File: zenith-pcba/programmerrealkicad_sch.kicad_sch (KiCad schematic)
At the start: 19 parts, among them SW1 G4R152312, U1 XC7K70T-FBG676, U3 CH347T, U4 AP63203WU, X1 SX5B8.000F1520F30

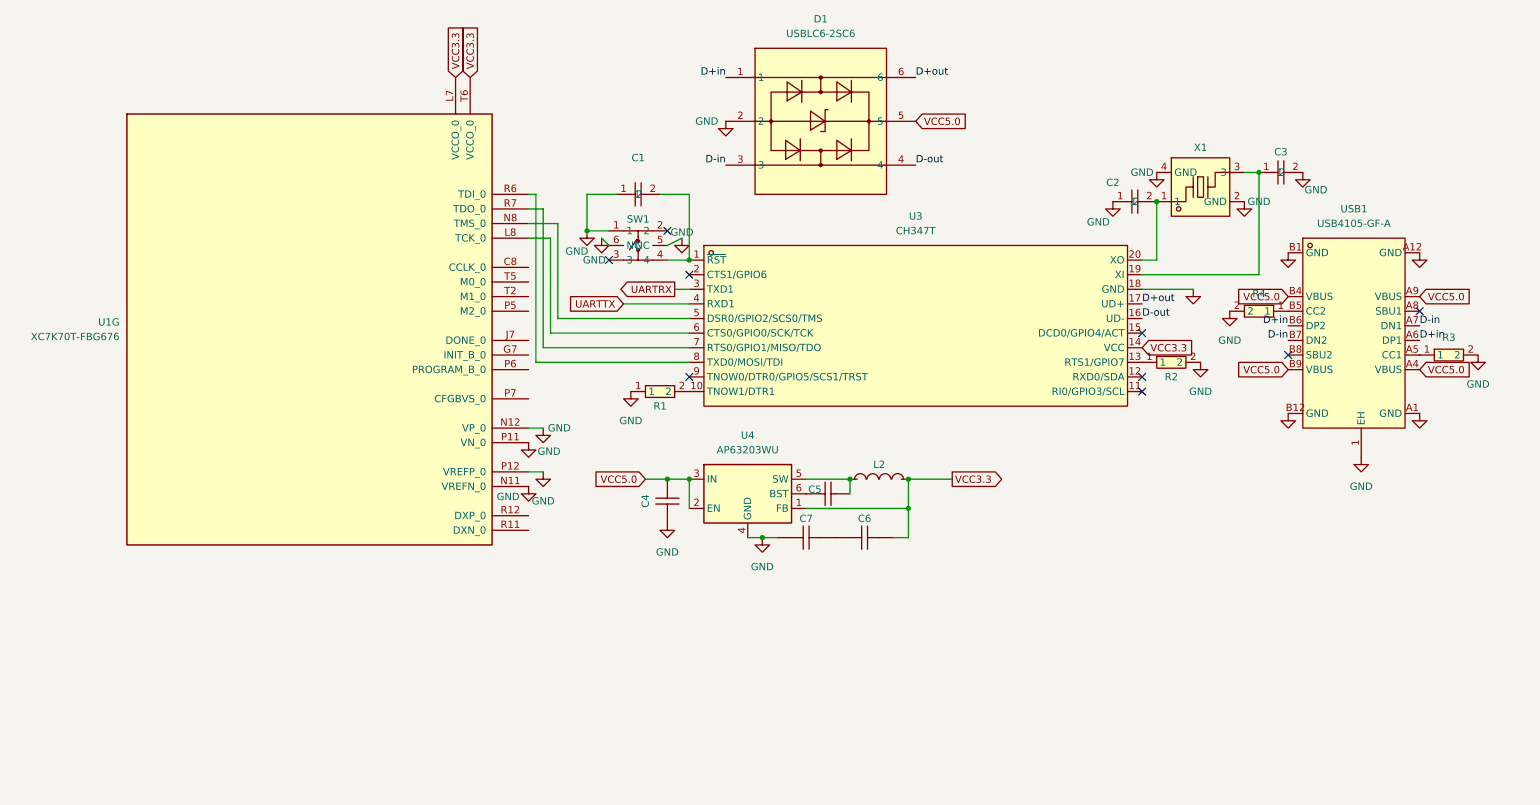
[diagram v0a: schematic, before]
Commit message: chore(pcba): clean up pages
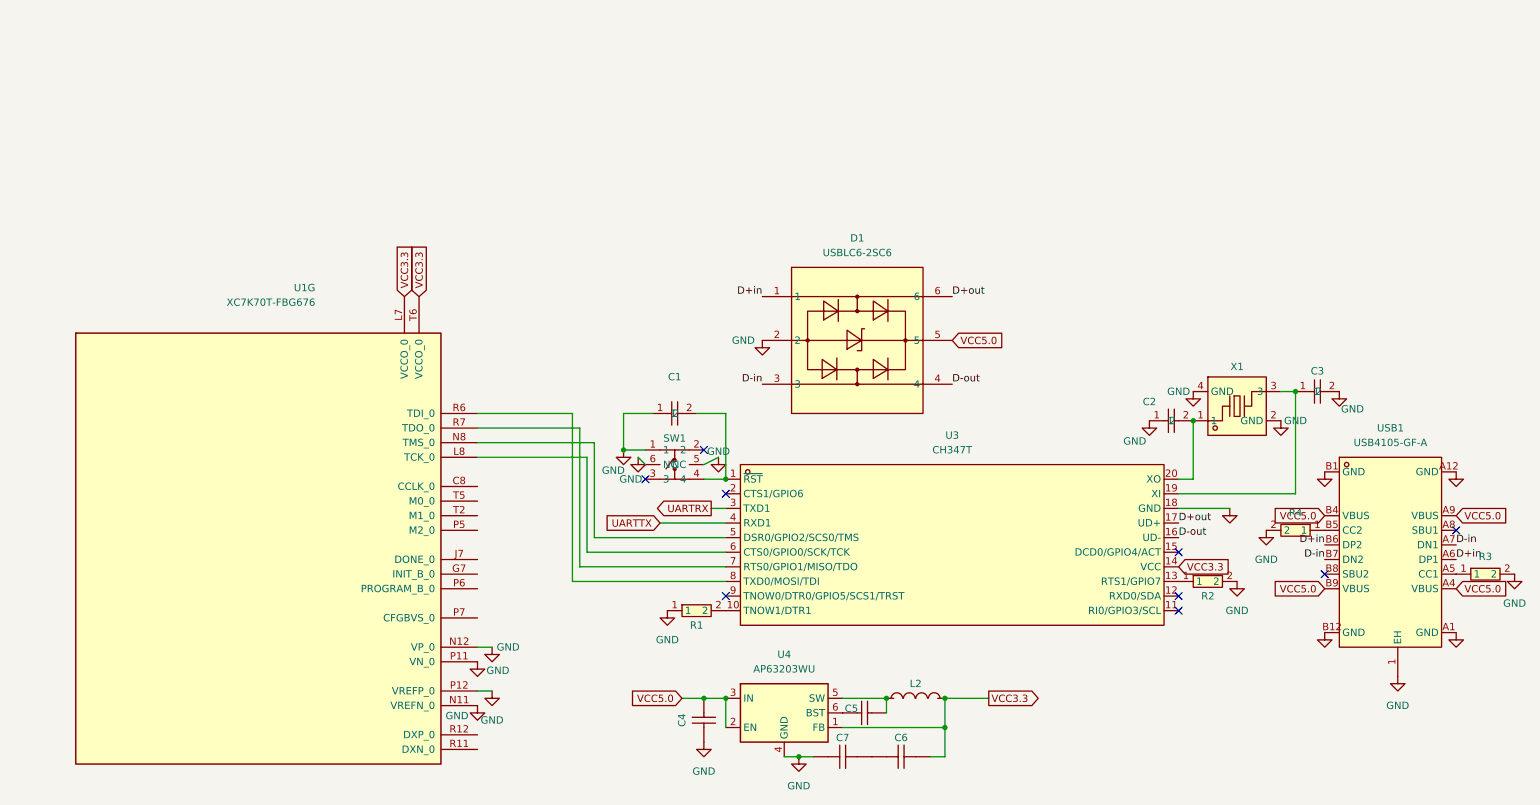
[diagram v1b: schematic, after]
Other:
- moved on the sheet: C1, C2, C3, C4, C5, C6, C7, D1, L2, R1, R2, R3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
